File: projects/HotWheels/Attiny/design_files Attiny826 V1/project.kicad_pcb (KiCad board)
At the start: 2 copper layers, 22 x 18 mm, 26 parts, among them J1 JST-SH, J2 BAT, J3 CHG, J4 UDPI, J5 HL, J6 TL, J7 FL, SW1 SW_SPDT, U1 ATtiny826

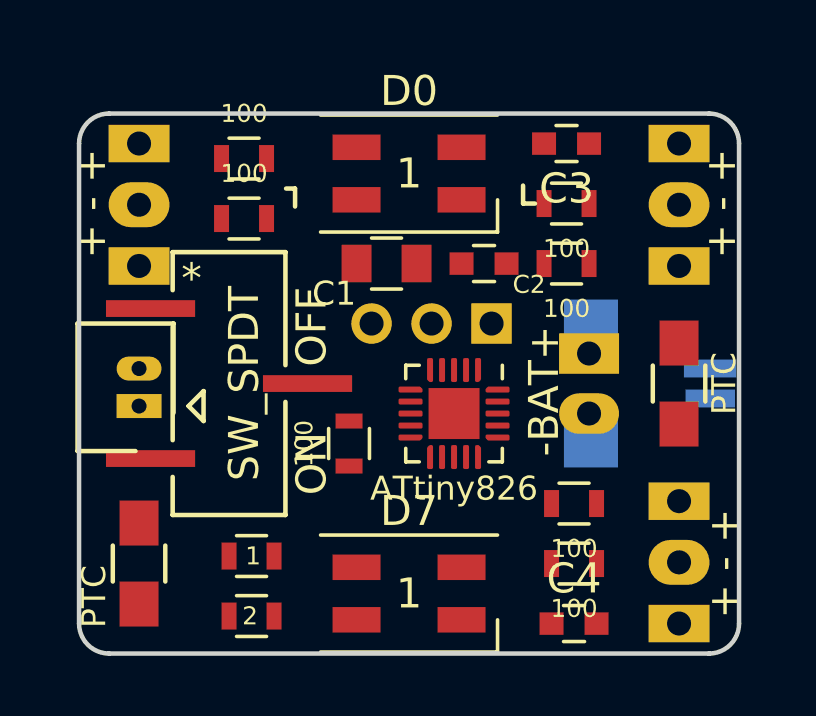
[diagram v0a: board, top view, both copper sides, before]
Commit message: Updates
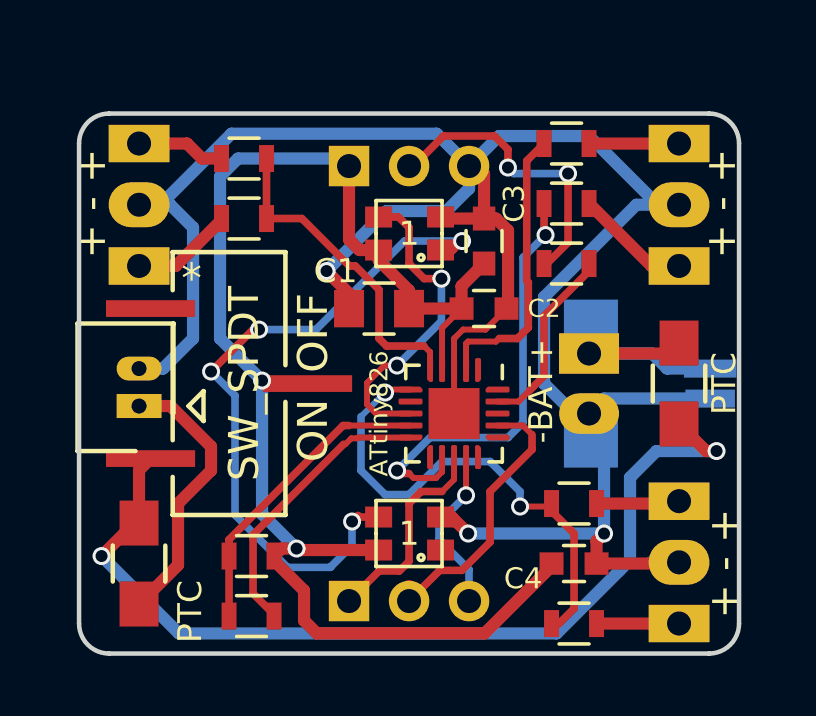
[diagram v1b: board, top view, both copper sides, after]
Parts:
- added J8: I2C, footprints:PinHeader_1x03_P2.00mm_Vertical, B.Cu at (137.0, 100.2)
- D0, D7: footprint LED_SMD:LED_SK6812MINI_PLCC4_3.5x3.5mm_P1.75mm -> footprints:WS2812B-2020
- J4: footprint Connector_PinHeader_2.00mm:PinHeader_1x03_P2.00mm_Vertical -> footprints:PinHeader_1x03_P2.00mm_Vertical
- moved R10 9.41 mm to (144.2, 89.0), turned to 180 degrees
- moved J4 7.08 mm to (137.0, 85.8), turned to 270 degrees
- moved C3 4.26 mm to (141.5, 88.2), turned to 90 degrees
- moved C4 2.00 mm to (144.5, 99.0)
- moved D0 2.00 mm to (139.0, 88.0)
- moved D7 2.00 mm to (139.0, 98.0)
- moved R4 2.00 mm to (144.5, 101.0)
- moved R6 2.00 mm to (144.2, 85.0)
- moved R7 2.00 mm to (144.2, 87.0)
- moved C1 1.52 mm to (138.0, 90.5)
- moved C2 1.50 mm to (141.5, 90.5)
- turned F1 to 90 degrees
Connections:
- D0 pad 3: /D4 -> /D3
- R1 pad 2: /A5 -> /D4
- R11 pad 1: /D1 -> /D0
- R2 pad 1: /A5 -> /D4
- R2 pad 2: GND -> /D5
- R4 pad 1: /D8 -> /D1
- R5 pad 1: /D9 -> /D1
- U1 pad 10: (no net) -> /D5
- U1 pad 13: /D8 -> /SDA
- U1 pad 14: /D9 -> /SCL
- U1 pad 17: (no net) -> /D12
- U1 pad 8: (no net) -> /D3
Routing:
- net GND: track 0.00 -> 79.4 mm, vias 0 -> 3
- net VCC: track 0.00 -> 47.4 mm, vias 0 -> 2
- net Net-(F1-Pad2): track 0.00 -> 31.3 mm, vias 0 -> 2
- net Net-(D0-Pad1): track 0.00 -> 22.8 mm, vias 0 -> 4
- net /D1: track 0.00 -> 16.7 mm, vias 0 -> 2
- net /D7: track 0.00 -> 14.7 mm, vias 0 -> 2
- net /D0: track 0.00 -> 10.8 mm
- net /D3: track 0.00 -> 10.7 mm, vias 0 -> 2
- net /D4: track 0.00 -> 10.2 mm
- net Net-(J4-Pad2): track 0.00 -> 9.98 mm, vias 0 -> 2
- net /D5: track 0.00 -> 9.59 mm
- net /D16: track 0.00 -> 9.58 mm
- net /D12: track 0.00 -> 9.46 mm
- net Net-(F1-Pad1): track 0.00 -> 9.20 mm
- net Net-(F2-Pad1): track 0.00 -> 8.42 mm
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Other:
- board text added: "D0"
- board text added: "D1"
- board text added: "D7-D16"
- board text added: "Rev 0.1 Apr 22"
- board text added: "c d"
- board text removed: "D1 - D4"
- board text removed: "D15-D16"
- board text removed: "D8 - D9"
- board text removed: "JST-SH"
- board text removed: "Rev 0.0 Mar 22"

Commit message: Updates
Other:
- board text added: "HW Attiny826 V1"
